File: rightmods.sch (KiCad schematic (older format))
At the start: 0 parts

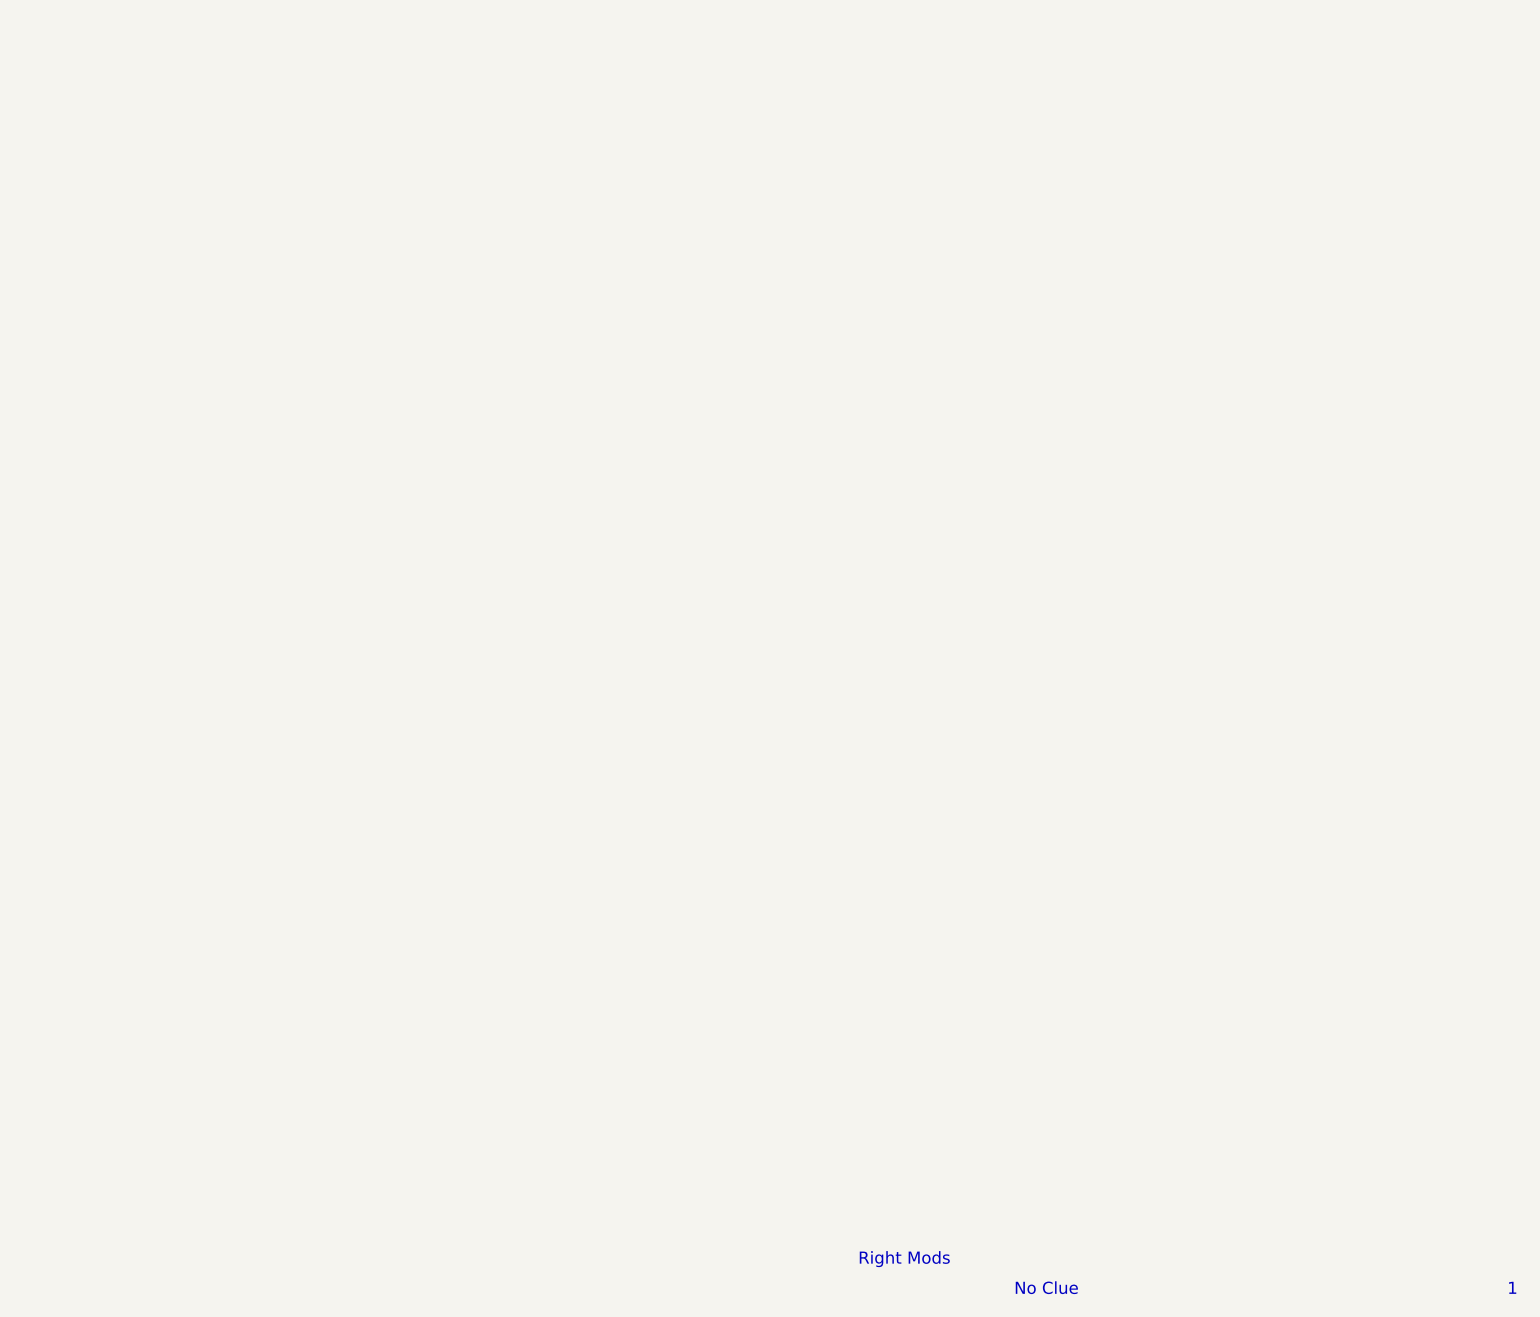
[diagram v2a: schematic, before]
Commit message: Added right mods
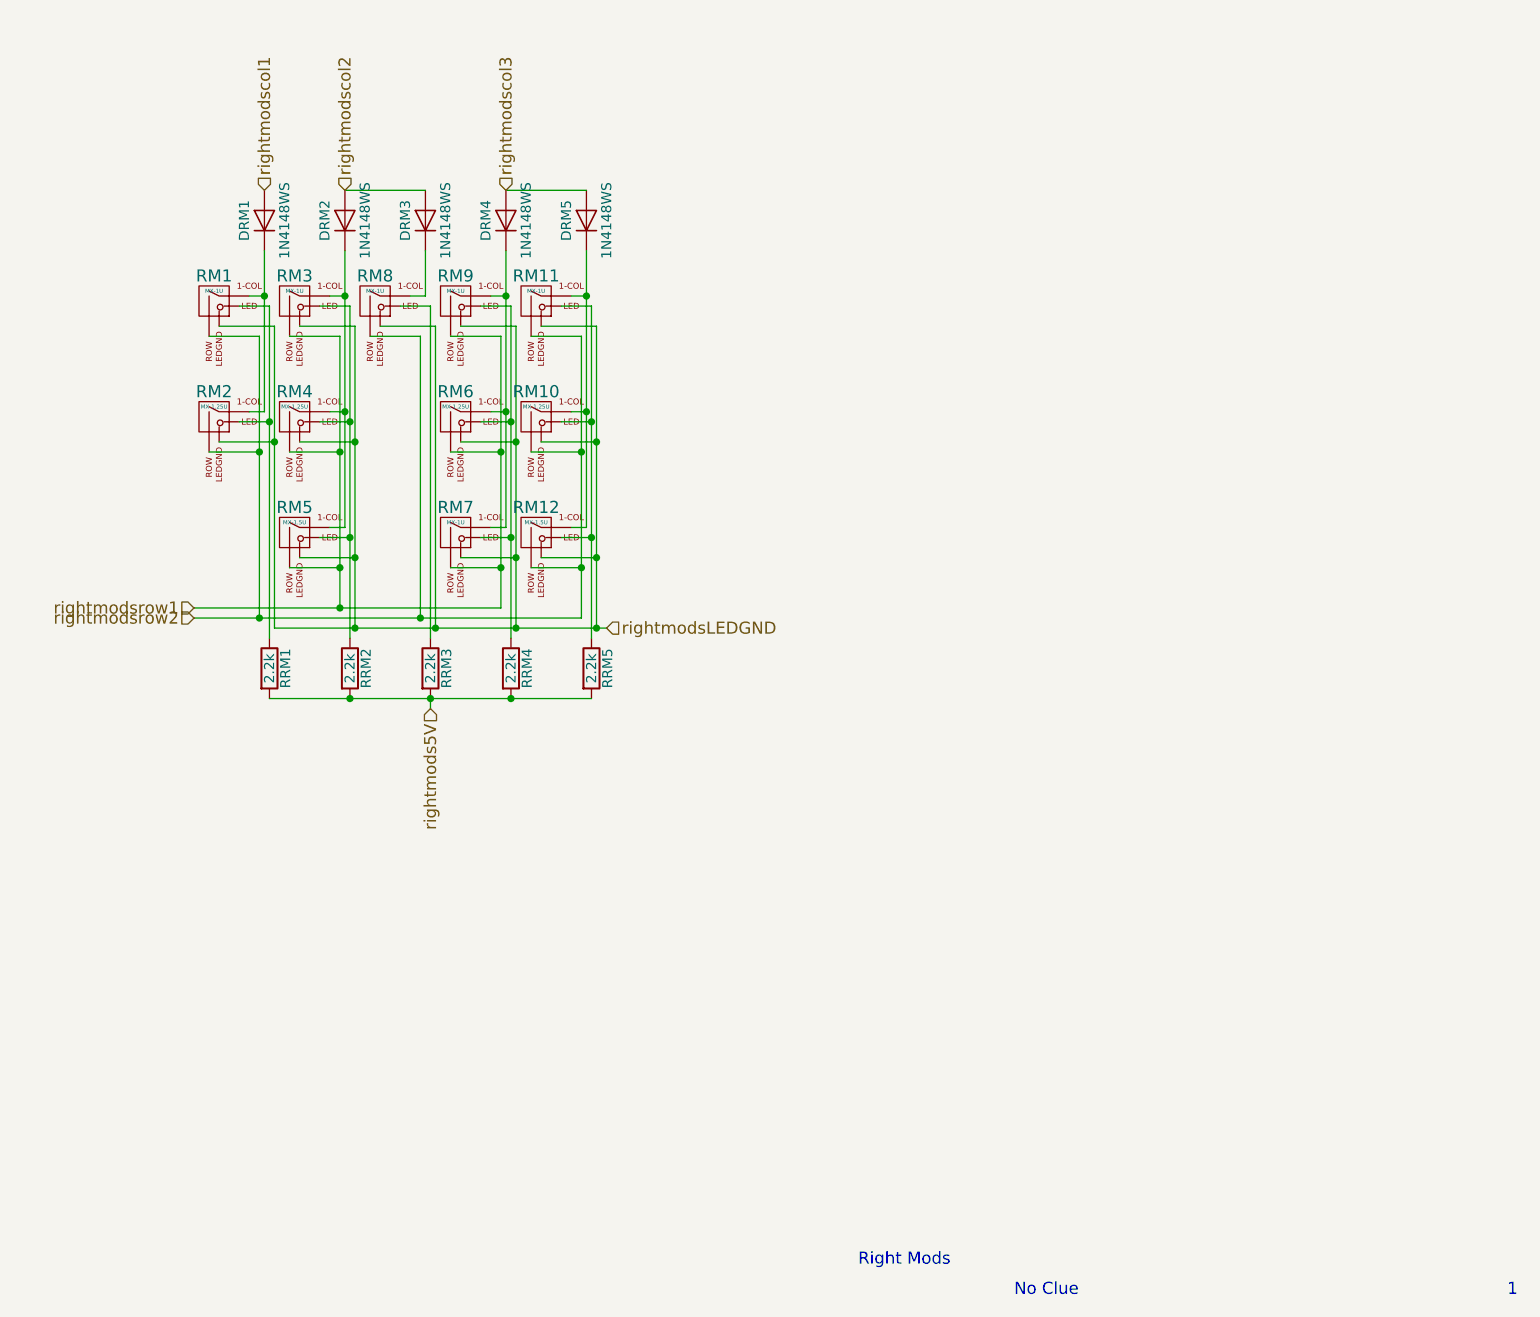
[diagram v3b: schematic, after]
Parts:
- added DRM1, DRM2, DRM3, DRM4, DRM5: 1N4148WS, symbol D
- added RM1, RM11, RM3, RM7, RM8, RM9: MX-1U, symbol MX-1U
- added RM10, RM2, RM4, RM6: MX-1.25U, symbol MX-1.25U
- added RM12, RM5: MX-1.5U, symbol MX-1.5U
- added RRM1, RRM2, RRM3, RRM4, RRM5: 2.2k, symbol R
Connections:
- new net: DRM1.1 (K), RM1.1 (COL), RM2.1 (COL)
- new net: RM1.3 (LED), RM2.3 (LED), RRM1.1
- new net: DRM2.1 (K), RM3.1 (COL), RM4.1 (COL), RM5.1 (COL)
- new net: RM3.3 (LED), RM4.3 (LED), RM5.3 (LED), RRM2.1
- new net: DRM4.1 (K), RM6.1 (COL), RM7.1 (COL), RM9.1 (COL)
- new net: RM6.3 (LED), RM7.3 (LED), RM9.3 (LED), RRM4.1
- new net: DRM3.1 (K), RM8.1 (COL)
- new net: RM8.3 (LED), RRM3.1
- new net: DRM5.1 (K), RM10.1 (COL), RM11.1 (COL), RM12.1 (COL)
- new net: RM10.3 (LED), RM11.3 (LED), RM12.3 (LED), RRM5.1
- new net rightmods5V: RRM1.2, RRM2.2, RRM3.2, RRM4.2, RRM5.2
- new net rightmodsLEDGND: RM1.4 (LEDGND), RM10.4 (LEDGND), RM11.4 (LEDGND), RM12.4 (LEDGND), RM2.4 (LEDGND), RM3.4 (LEDGND), RM4.4 (LEDGND), RM5.4 (LEDGND), RM6.4 (LEDGND), RM7.4 (LEDGND), RM8.4 (LEDGND), RM9.4 (LEDGND)
- new net rightmodscol1: DRM1.2 (A)
- new net rightmodscol2: DRM2.2 (A), DRM3.2 (A)
- new net rightmodscol3: DRM4.2 (A), DRM5.2 (A)
- new net rightmodsrow1: RM3.2 (ROW), RM4.2 (ROW), RM5.2 (ROW), RM6.2 (ROW), RM7.2 (ROW), RM9.2 (ROW)
- new net rightmodsrow2: RM1.2 (ROW), RM10.2 (ROW), RM11.2 (ROW), RM12.2 (ROW), RM2.2 (ROW), RM8.2 (ROW)
